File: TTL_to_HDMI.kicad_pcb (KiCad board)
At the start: 2 copper layers, 74 x 66.5 mm, 42 parts, among them J1 Conn_01x32_Pin, J2 Conn_01x32_Pin, Q2 Q_NPN_BEC, U1 1x50, U2 1x50, U3 74LVX541, U5 NANO_9K, U6 74LVX541, U7 74LVX541, U8 74LVX541

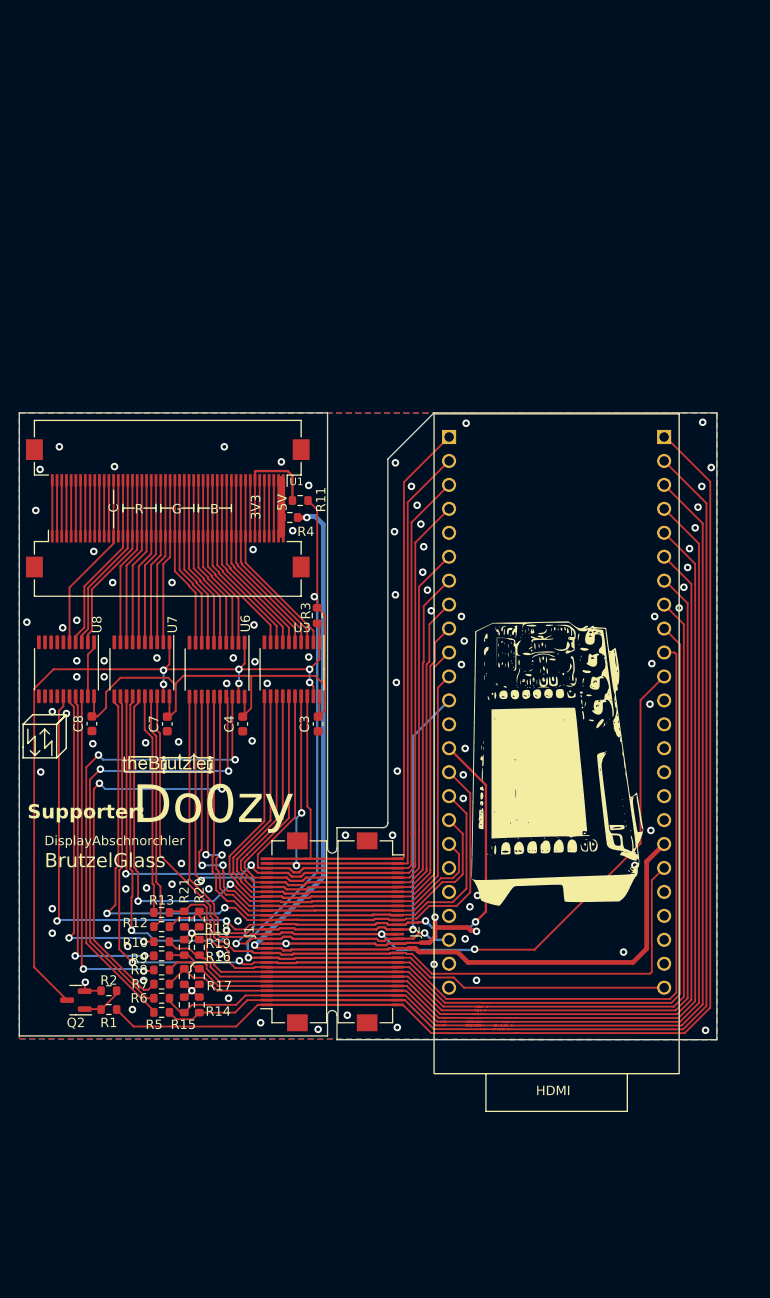
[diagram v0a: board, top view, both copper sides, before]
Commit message: Update Final stade
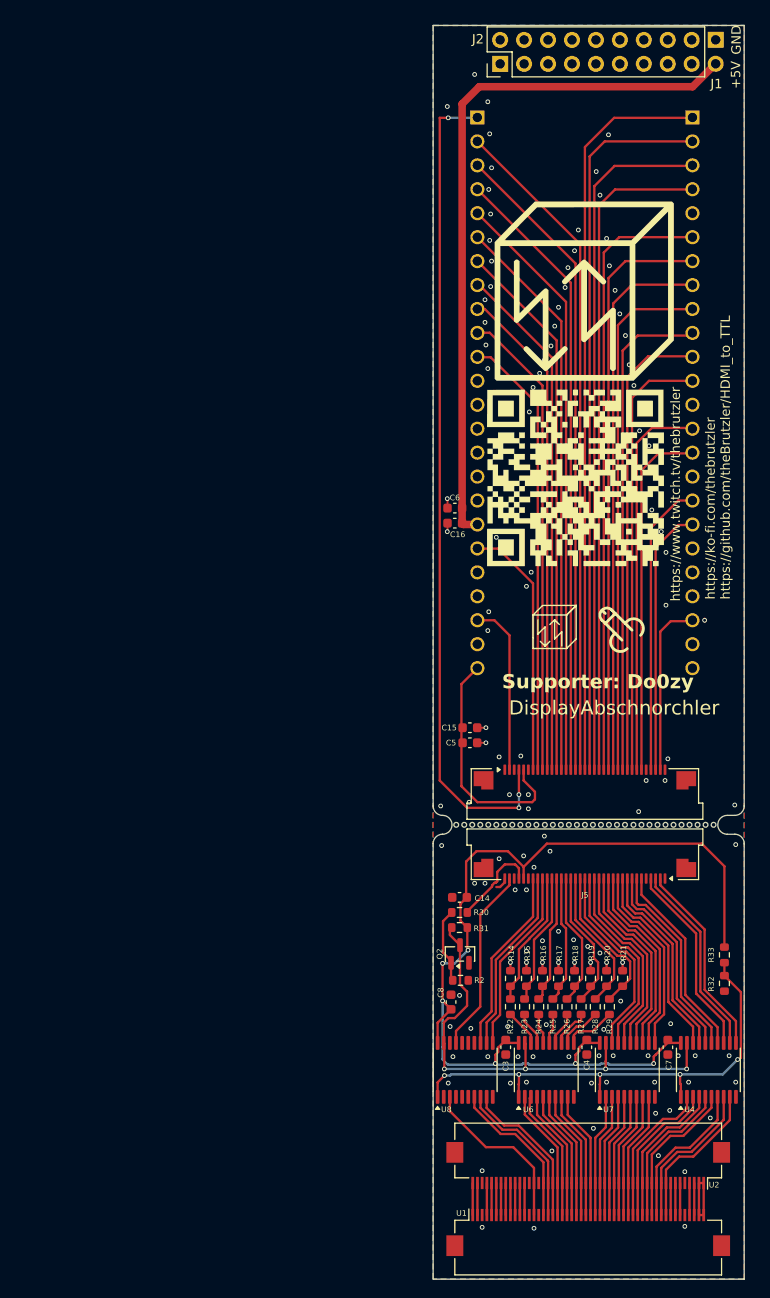
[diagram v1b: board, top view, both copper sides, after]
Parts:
- removed the G*** at (91.8, 109.1)
- removed the G*** at (133.0, 109.0)
- removed the G*** at (118.2, 109.4)
- removed the G*** at (133.0, 109.3)
- removed the G*** at (133.8, 132.8)
- removed the G*** at (133.9, 83.2)
- removed R1, R10, R12, R13, R3, R5, R6, R7, R8, R9: 10K, Resistor_SMD:R_0603_1608Metric
- removed R11, R4: 0, Resistor_SMD:R_0603_1608Metric
- removed U3: 74LVX541, Package_SO:TSSOP-20_4.4x6.5mm_P0.65mm
- added C14: 10u, Capacitor_SMD:C_0603_1608Metric, F.Cu at (122.7, 123.3)
- added C15: 10u, Capacitor_SMD:C_0603_1608Metric, F.Cu at (123.8, 105.3)
- added C16: 10u, Capacitor_SMD:C_0603_1608Metric, F.Cu at (122.2, 82.0)
- added C5: 100n, Capacitor_SMD:C_0603_1608Metric, F.Cu at (123.8, 106.9)
- added C6: 100n, Capacitor_SMD:C_0603_1608Metric, F.Cu at (122.2, 83.6)
- added G***: LOGO, theBrutzler:Symbol_kurzschlussblog_20mm, F.Cu at (135.9, 59.1)
- added G***: LOGO, LOGO, F.Cu at (134.7, 78.7)
- added J3: Conn_01x35_Pin, Connector_FFC-FPC:Amphenol_F32Q-1A7x1-11035_1x35-1MP_P0.5mm_Horizontal, F.Cu at (136.0, 112.7)
- added J5: Conn_01x35_Pin, Connector_FFC-FPC:Amphenol_F32Q-1A7x1-11035_1x35-1MP_P0.5mm_Horizontal, F.Cu at (136.0, 118.4)
- added R22: 1K, Resistor_SMD:R_0603_1608Metric, F.Cu at (128.1, 134.9)
- added R23: 1K, Resistor_SMD:R_0603_1608Metric, F.Cu at (129.6, 134.9)
- added R24: 1K, Resistor_SMD:R_0603_1608Metric, F.Cu at (131.1, 134.9)
- added R25: 1K, Resistor_SMD:R_0603_1608Metric, F.Cu at (132.6, 134.9)
- added R26: 1K, Resistor_SMD:R_0603_1608Metric, F.Cu at (134.1, 134.9)
- added R27: 1K, Resistor_SMD:R_0603_1608Metric, F.Cu at (135.6, 134.9)
- added R28: 1K, Resistor_SMD:R_0603_1608Metric, F.Cu at (137.1, 134.9)
- added R29: 1K, Resistor_SMD:R_0603_1608Metric, F.Cu at (138.6, 134.9)
- added R30: 1K, Resistor_SMD:R_0603_1608Metric, F.Cu at (122.7, 124.9)
- added R31: 1K, Resistor_SMD:R_0603_1608Metric, F.Cu at (122.7, 126.5)
- added R32: 1K, Resistor_SMD:R_0603_1608Metric, F.Cu at (150.8, 132.4)
- added R33: 1K, Resistor_SMD:R_0603_1608Metric, F.Cu at (150.8, 129.4)
- added REF**: BreakLine_11h_D0.5mm_P0.85mm, Panelization:BreakLine_11h_D0.5mm_P0.85mm, F.Cu at (126.6, 115.6)
- added REF**: BreakLine_11h_D0.5mm_P0.85mm, Panelization:BreakLine_11h_D0.5mm_P0.85mm, F.Cu at (136.0, 115.6)
- added REF**: BreakLine_11h_D0.5mm_P0.85mm, Panelization:BreakLine_11h_D0.5mm_P0.85mm, F.Cu at (145.4, 115.6)
- added REF**: penoid, theBrutzler:penoid, F.Cu at (139.4, 94.5)
- added U4: 74HC245, Package_SO:TSSOP-20_4.4x6.5mm_P0.65mm, F.Cu at (149.1, 141.6)
- J1: value Conn_01x32_Pin -> Conn_01x02_Socket; footprint Connector_FFC-FPC:Hirose_FH12-32S-0.5SH_1x32-1MP_P0.50mm_Horizontal -> Connector_PinHeader_2.54mm:PinHeader_1x02_P2.54mm_Vertical; moved to B.Cu
- J2: value Conn_01x32_Pin -> ONLY DUMMY; footprint Connector_FFC-FPC:Hirose_FH12-32S-0.5SH_1x32-1MP_P0.50mm_Horizontal -> Connector_PinHeader_2.54mm:PinHeader_2x09_P2.54mm_Vertical
- R14, R15, R16, R17, R18, R19, R20, R21: value 10K -> 1K
- U5: moved to B.Cu
- U6, U7, U8: value 74LVX541 -> 74HC245
- moved J1 105.1 mm to (149.9, 32.3), turned to 180 degrees
- moved U1 93.0 mm to (136.3, 158.8), turned to 0 degrees
- moved J2 92.9 mm to (127.0, 34.9), turned to 90 degrees
- moved U2 78.7 mm to (136.3, 151.8), turned to 180 degrees
- moved U7 66.8 mm to (140.5, 141.6), turned to 90 degrees
- moved C7 63.2 mm to (144.8, 139.2)
- moved U8 60.0 mm to (123.3, 141.6), turned to 90 degrees
- moved SM3 55.3 mm to (130.5, 96.9)
- moved U6 55.0 mm to (131.9, 141.6), turned to 90 degrees
- moved C4 50.1 mm to (136.2, 139.2)
- moved C8 48.2 mm to (121.8, 134.4), turned to -90 degrees
- moved R21 46.9 mm to (140.0, 131.9), turned to -90 degrees
- moved R20 43.7 mm to (138.3, 131.9), turned to -90 degrees
- moved R19 41.6 mm to (136.6, 131.9)
- moved R18 41.5 mm to (134.9, 131.9)
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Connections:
- net VCC renamed Net-(U1-Pad7)
- J1 pad 1: /32 -> GND
- J1 pad 2: /31 -> +5V
- J2 pad 1: F_DE -> unconnected-(J2-Pin_1-Pad1)
- J2 pad 10: F_R7 -> unconnected-(J2-Pin_10-Pad10)
- J2 pad 11: F_G5 -> unconnected-(J2-Pin_11-Pad11)
- J2 pad 12: F_G6 -> unconnected-(J2-Pin_12-Pad12)
- J2 pad 13: F_G7 -> unconnected-(J2-Pin_13-Pad13)
- J2 pad 14: F_R3 -> unconnected-(J2-Pin_14-Pad14)
- J2 pad 15: F_CLK -> unconnected-(J2-Pin_15-Pad15)
- J2 pad 16: F_R6 -> unconnected-(J2-Pin_16-Pad16)
- J2 pad 17: F_G3 -> (no net)
- J2 pad 18: F_G4 -> (no net)
- J2 pad 2: F_VS -> unconnected-(J2-Pin_2-Pad2)
- J2 pad 3: F_HS -> unconnected-(J2-Pin_3-Pad3)
- J2 pad 4: F_R5 -> unconnected-(J2-Pin_4-Pad4)
- J2 pad 5: F_B7 -> unconnected-(J2-Pin_5-Pad5)
- J2 pad 6: F_B6 -> unconnected-(J2-Pin_6-Pad6)
- J2 pad 7: F_B5 -> unconnected-(J2-Pin_7-Pad7)
- J2 pad 8: F_B4 -> unconnected-(J2-Pin_8-Pad8)
- J2 pad 9: F_B3 -> unconnected-(J2-Pin_9-Pad9)
- Q2 pad 3: F_OE1 -> F_OE
- R14 pad 2: /31 -> /10
- R15 pad 2: /30 -> /11
- R16 pad 2: /29 -> /12
- R17 pad 2: /28 -> /13
- R18 pad 2: /27 -> /14
- R19 pad 2: /26 -> /15
- R20 pad 2: /25 -> /16
- R21 pad 2: /24 -> /17
- U1 pad 1: Net-(R4-Pad1) -> Net-(U1-Pad1)
- U1 pad 10: VS -> Net-(U1-Pad10)
- U1 pad 11: HS -> Net-(U1-Pad11)
- U1 pad 12: B7 -> Net-(U1-Pad12)
- U1 pad 13: B6 -> GND
- U1 pad 14: B5 -> CLK
- U1 pad 15: B4 -> GND
- U1 pad 16: B3 -> R0
- U1 pad 17: B2 -> R1
- U1 pad 18: B1 -> R2
- U1 pad 19: B0 -> R3
- U1 pad 2: Net-(R4-Pad1) -> Net-(U1-Pad2)
- U1 pad 20: G7 -> R4
- U1 pad 21: G6 -> R5
- U1 pad 22: G5 -> R6
- U1 pad 23: G4 -> R7
- U1 pad 24: G3 -> G0
- U1 pad 25: G2 -> G1
- U1 pad 26: G1 -> G2
- U1 pad 27: G0 -> G3
- U1 pad 28: R7 -> G4
- U1 pad 29: R6 -> G5
- U1 pad 3: Net-(U1-Pad3) -> GND
- U1 pad 30: R5 -> G6
- U1 pad 31: R4 -> G7
- U1 pad 32: R3 -> B0
- U1 pad 33: R2 -> B1
- U1 pad 34: R1 -> B2
- U1 pad 35: R0 -> B3
- U1 pad 36: GND -> B4
- U1 pad 37: CLK -> B5
- U1 pad 38: GND -> B6
- U1 pad 39: Net-(U1-Pad39) -> B7
- U1 pad 40: Net-(U1-Pad40) -> HS
- U1 pad 41: Net-(U1-Pad41) -> VS
- U1 pad 42: Net-(U1-Pad42) -> DE
- U1 pad 46: Net-(U1-Pad46) -> GND
- U1 pad 48: GND -> Net-(U1-Pad48)
- U1 pad 49: Net-(U1-Pad49) -> V_BLK
- U1 pad 5: GND -> Net-(U1-Pad5)
- U1 pad 50: Net-(U1-Pad50) -> V_BLK
- U1 pad 9: DE -> Net-(U1-Pad9)
- U2 pad 1: Net-(U1-Pad50) -> V_BLK
- U2 pad 10: Net-(U1-Pad41) -> VS
- U2 pad 11: Net-(U1-Pad40) -> HS
- U2 pad 12: Net-(U1-Pad39) -> B7
- U2 pad 13: GND -> B6
- U2 pad 14: CLK -> B5
- U2 pad 15: GND -> B4
- U2 pad 16: R0 -> B3
- U2 pad 17: R1 -> B2
- U2 pad 18: R2 -> B1
- U2 pad 19: R3 -> B0
- U2 pad 2: Net-(U1-Pad49) -> V_BLK
- U2 pad 20: R4 -> G7
- U2 pad 21: R5 -> G6
- U2 pad 22: R6 -> G5
- U2 pad 23: R7 -> G4
- U2 pad 24: G0 -> G3
- U2 pad 25: G1 -> G2
- U2 pad 26: G2 -> G1
- U2 pad 27: G3 -> G0
- U2 pad 28: G4 -> R7
- U2 pad 29: G5 -> R6
- U2 pad 3: GND -> Net-(U1-Pad48)
- U2 pad 30: G6 -> R5
- U2 pad 31: G7 -> R4
- U2 pad 32: B0 -> R3
- U2 pad 33: B1 -> R2
- U2 pad 34: B2 -> R1
- U2 pad 35: B3 -> R0
- U2 pad 36: B4 -> GND
- U2 pad 37: B5 -> CLK
- U2 pad 38: B6 -> GND
- U2 pad 39: B7 -> Net-(U1-Pad12)
- U2 pad 40: HS -> Net-(U1-Pad11)
- U2 pad 41: VS -> Net-(U1-Pad10)
- U2 pad 42: DE -> Net-(U1-Pad9)
- U2 pad 46: GND -> Net-(U1-Pad5)
- U2 pad 48: Net-(U1-Pad3) -> GND
- U2 pad 49: Net-(R4-Pad1) -> Net-(U1-Pad2)
- U2 pad 5: Net-(U1-Pad46) -> GND
- U2 pad 50: Net-(R4-Pad1) -> Net-(U1-Pad1)
- U2 pad 9: Net-(U1-Pad42) -> DE
- U5 pad 1: F_DE -> F_G3
- U5 pad 11: F_R7 -> F_B4
- U5 pad 12: F_R6 -> F_B5
- U5 pad 14: F_CLK -> F_B6
- U5 pad 15: F_R3 -> F_B7
- U5 pad 16: F_G7 -> unconnected-(U5-IOB41B-Pad16)
- U5 pad 17: F_G6 -> F_HS
- U5 pad 18: F_G5 -> F_VS
- U5 pad 2: F_VS -> F_G4
- U5 pad 22: F_G4 -> F_DE
- U5 pad 27: unconnected-(U5-IOB15B-Pad27) -> F_CLK
- U5 pad 3: F_HS -> F_G5
- U5 pad 30: F_G2 -> F_R0
- U5 pad 38: F_G3 -> F_R1
- U5 pad 39: F_R4 -> F_R2
- U5 pad 4: F_R5 -> F_G6
- U5 pad 40: /24 -> /10
- U5 pad 41: /25 -> /11
- U5 pad 42: /26 -> /12
- U5 pad 43: /27 -> /13
- U5 pad 44: /28 -> /14
- U5 pad 45: /29 -> /15
- U5 pad 46: /30 -> /16
- U5 pad 47: /31 -> /17
- U5 pad 48: /32 -> /4
- U5 pad 6: F_B7 -> F_G7
- U5 pad 7: F_B6 -> F_B0
- U5 pad 8: F_B5 -> F_B1
- U5 pad 9: F_B4 -> F_B2
- U6 pad 1: F_OE1 -> F_DIR
- U6 pad 11: F_G3 -> F_G2
- U6 pad 12: F_G4 -> F_G1
- U6 pad 13: F_G5 -> F_G0
- U6 pad 14: F_G6 -> F_R7
- U6 pad 15: F_G7 -> F_R6
- U6 pad 16: F_B0 -> F_R5
- U6 pad 17: F_B1 -> F_R4
- U6 pad 18: F_B2 -> F_R3
- U6 pad 19: F_OE1 -> F_OE
- U6 pad 2: B2 -> R3
- U6 pad 3: B1 -> R4
- U6 pad 4: B0 -> R5
- U6 pad 5: G7 -> R6
- U6 pad 6: G6 -> R7
- U6 pad 7: G5 -> G0
- U6 pad 8: G4 -> G1
- U6 pad 9: G3 -> G2
- U7 pad 1: F_OE1 -> F_DIR
- U7 pad 11: F_R3 -> F_B2
- U7 pad 12: F_R4 -> F_B1
- U7 pad 13: F_R5 -> F_B0
- U7 pad 14: F_R6 -> F_G7
- U7 pad 15: F_R7 -> F_G6
- U7 pad 16: F_G0 -> F_G5
- U7 pad 17: F_G1 -> F_G4
- U7 pad 18: F_G2 -> F_G3
- U7 pad 19: F_OE1 -> F_OE
- U7 pad 2: G2 -> G3
- U7 pad 3: G1 -> G4
- U7 pad 4: G0 -> G5
- U7 pad 5: R7 -> G6
- U7 pad 6: R6 -> G7
- U7 pad 7: R5 -> B0
- U7 pad 8: R4 -> B1
- U7 pad 9: R3 -> B2
- U8 pad 1: F_OE1 -> F_DIR
- U8 pad 11: unconnected-(U8-Y7-Pad11) -> F_R2
- U8 pad 12: unconnected-(U8-Y6-Pad12) -> F_R1
- U8 pad 13: unconnected-(U8-Y5-Pad13) -> F_R0
- U8 pad 15: F_CLK -> unconnected-(U8-B3-Pad15)
- U8 pad 16: F_R0 -> unconnected-(U8-B2-Pad16)
- U8 pad 17: F_R1 -> F_CLK
- U8 pad 18: F_R2 -> unconnected-(U8-B0-Pad18)
- U8 pad 19: F_OE1 -> F_OE
- U8 pad 2: R2 -> GND
- U8 pad 3: R1 -> CLK
- U8 pad 4: R0 -> GND
- U8 pad 5: CLK -> GND
- U8 pad 7: GND -> R0
- U8 pad 8: GND -> R1
- U8 pad 9: GND -> R2
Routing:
- net /32: track 129.7 -> 0.00 mm
- net F_R4: track 126.2 -> 3.56 mm, vias 2 -> 0
- net /31: track 120.1 -> 0.00 mm
- net /30: track 117.2 -> 0.00 mm
- net /29: track 114.0 -> 0.00 mm
- net /28: track 110.4 -> 0.00 mm
- net /27: track 107.1 -> 0.00 mm
- net /25: track 104.9 -> 0.00 mm
- net /26: track 104.1 -> 0.00 mm
- net /24: track 101.2 -> 0.00 mm
- net /4: track 0.00 -> 97.5 mm, vias 0 -> 3
- net F_OE1: track 91.0 -> 0.00 mm, vias 6 -> 0
- net /17: track 0.00 -> 87.5 mm
- net F_R5: track 90.4 -> 3.21 mm, vias 2 -> 0
- net /16: track 0.00 -> 83.7 mm
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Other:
- board size 74 x 66.5 mm -> 33 x 133 mm
- board text added: "+5V"
- board text added: "GND"
- board text added: "Supporter: Do0zy"
- board text added: "https://github.com/theBrutzler/HDMI_to_TTL"
- board text added: "https://ko-fi.com/thebrutzler"
- board text added: "https://www.twitch.tv/thebrutzler"
- board text removed: "3V3"
- board text removed: "5V"
- board text removed: "B"
- board text removed: "BrutzelGlass"
- board text removed: "C"
- board text removed: "Do0zy"
- board text removed: "G"
- board text removed: "R"
- board text removed: "Supporter:"
